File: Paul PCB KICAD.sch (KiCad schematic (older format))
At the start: 160 parts, among them SW1 SW_Push, U1 ATmega32U4-AU, Y1 16MHz

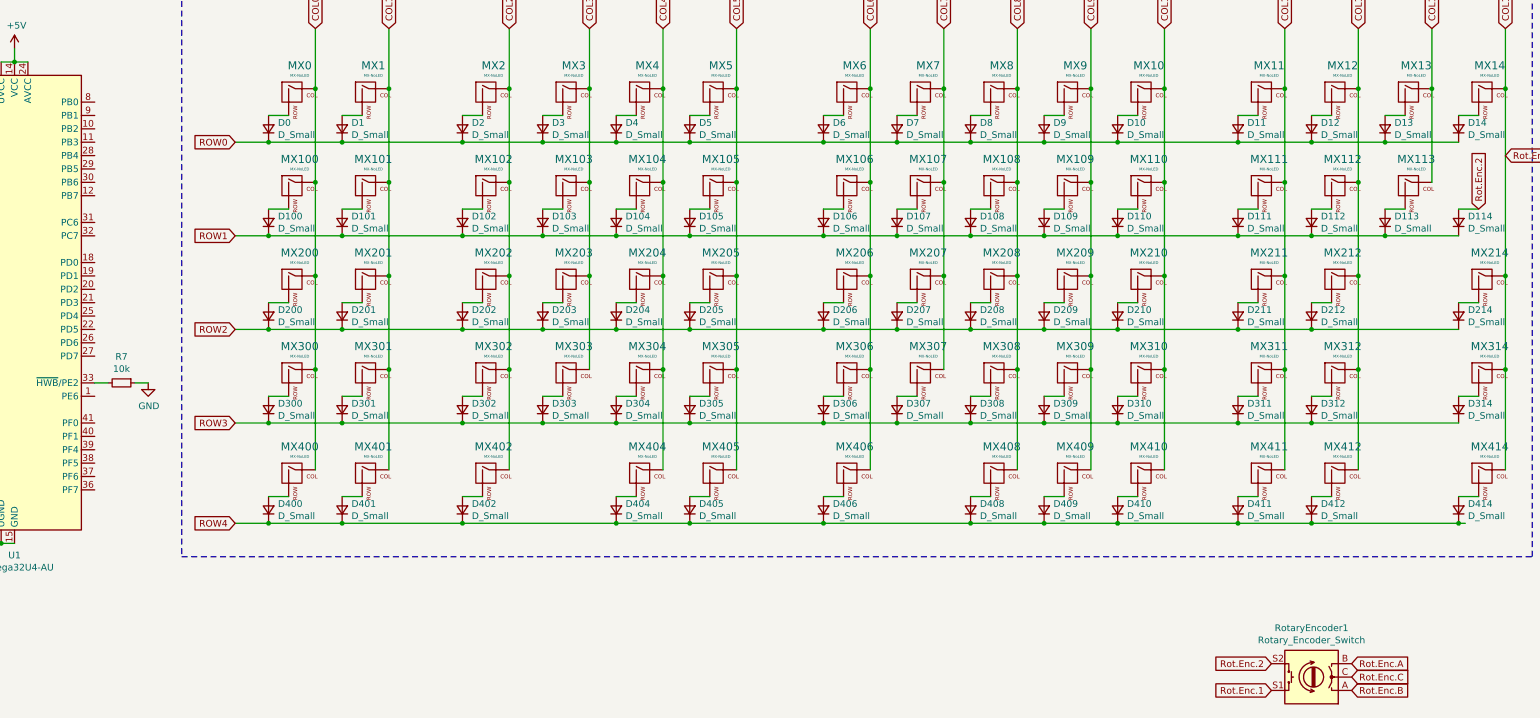
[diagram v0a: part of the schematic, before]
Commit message: Finished V1.0
I think it may be done
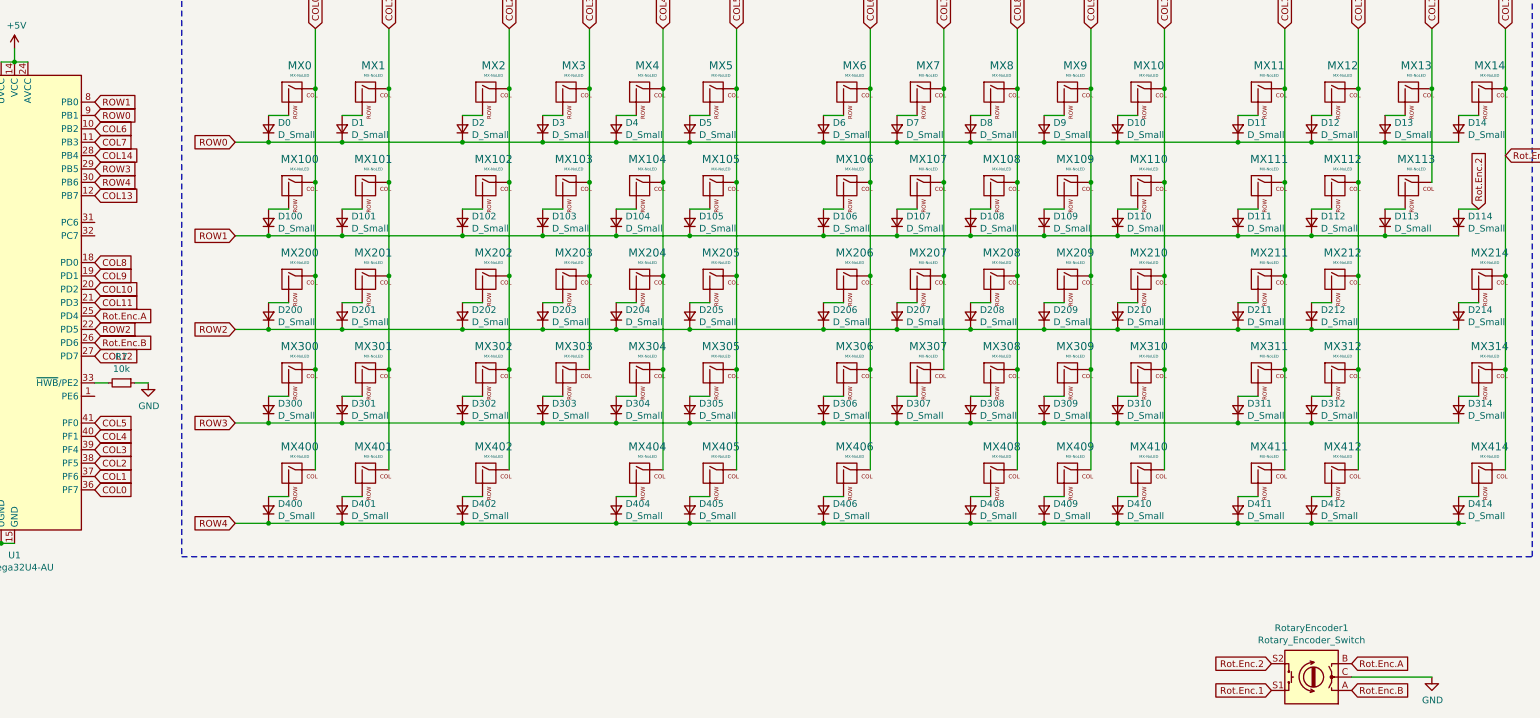
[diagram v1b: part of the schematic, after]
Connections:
- net Rot.Enc.C is gone; now on net GND: RotaryEncoder1.C
- net COL0: now also U1.36 (PF7)
- net COL1: now also U1.37 (PF6)
- net COL10: now also U1.20 (PD2)
- net COL11: now also U1.21 (PD3)
- net COL12: now also U1.27 (PD7)
- net COL13: now also U1.12 (PB7)
- net COL14: now also U1.28 (PB4)
- net COL2: now also U1.38 (PF5)
- net COL3: now also U1.39 (PF4)
- net COL4: now also U1.40 (PF1)
- net COL5: now also U1.41 (PF0)
- net COL6: now also U1.10 (PB2)
- net COL7: now also U1.11 (PB3)
- net COL8: now also U1.18 (PD0)
- net COL9: now also U1.19 (PD1)
- net ROW0: now also U1.9 (PB1)
- net ROW1: now also U1.8 (PB0)
- net ROW2: now also U1.22 (PD5)
- net ROW3: now also U1.29 (PB5)
- net ROW4: now also U1.30 (PB6)
- net Rot.Enc.A: now also U1.25 (PD4)
- net Rot.Enc.B: now also U1.26 (PD6)
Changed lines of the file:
@@
 	5700 1150 5700 5450
-Wire Notes Line
-	5700 5450 15800 5450
 Wire Notes Line
 	15800 5450 15800 1150
@@
 Text GLabel 14450 6250 2    50   Input ~ 0
 Rot.Enc.A
-Text GLabel 14450 6350 2    50   Input ~ 0
-Rot.Enc.C
 Text GLabel 14450 6450 2    50   Input ~ 0
 Rot.Enc.B
@@
 Wire Wire Line
 	11600 5200 12150 5200
+Text GLabel 5050 4950 2    50   Input ~ 0
+COL0
+Text GLabel 5050 4850 2    50   Input ~ 0
+COL1
+Text GLabel 5050 4750 2    50   Input ~ 0
+COL2
+Text GLabel 5050 4650 2    50   Input ~ 0
+COL3
+Text GLabel 5050 4550 2    50   Input ~ 0
+COL4
+Text GLabel 5050 4450 2    50   Input ~ 0
+COL5
+Text GLabel 5050 2050 2    50   Input ~ 0
+ROW1
+Text GLabel 5050 2150 2    50   Input ~ 0
+ROW0
+Text GLabel 5050 2250 2    50   Input ~ 0
+COL6
+Text GLabel 5050 2350 2    50   Input ~ 0
+COL7
+Text GLabel 5050 3250 2    50   Input ~ 0
+COL8
+Text GLabel 5050 3350 2    50   Input ~ 0
+COL9
+Text GLabel 5050 3450 2    50   Input ~ 0
+COL10
+Text GLabel 5050 3550 2    50   Input ~ 0
+COL11
+Text GLabel 5050 3750 2    50   Input ~ 0
+ROW2
+Text GLabel 5050 3950 2    50   Input ~ 0
+COL12
+Text GLabel 5050 2750 2    50   Input ~ 0
+COL13
+Text GLabel 5050 2450 2    50   Input ~ 0
+COL14
+Text GLabel 5050 2550 2    50   Input ~ 0
+ROW3
+Wire Notes Line
+	5700 5450 15800 5450
+Text GLabel 5050 2650 2    50   Input ~ 0
+ROW4
+Text GLabel 5050 3650 2    50   Input ~ 0
+Rot.Enc.A
+Text GLabel 5050 3850 2    50   Input ~ 0
+Rot.Enc.B
+$Comp
+L power:GND #PWR?
+U 1 1 612905BE
+P 15050 6350
+F 0 "#PWR?" H 15050 6100 50  0001 C CNN
+F 1 "GND" H 15055 6177 50  0000 C CNN
+F 2 "" H 15050 6350 50  0001 C CNN
+F 3 "" H 15050 6350 50  0001 C CNN
+	1    15050 6350
+	1    0    0    -1
+$EndComp
+Wire Wire Line
+	14450 6350 15050 6350
 $EndSCHEMATC
